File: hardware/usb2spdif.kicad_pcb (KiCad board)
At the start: 2 copper layers, 23 x 20.5 mm, 18 parts, among them J1 USB_C_Receptacle_USB2.0_16P, U1 RP2040, U2 W25Q16JVSS, U3 AP130-33Y, Y1 12MHz

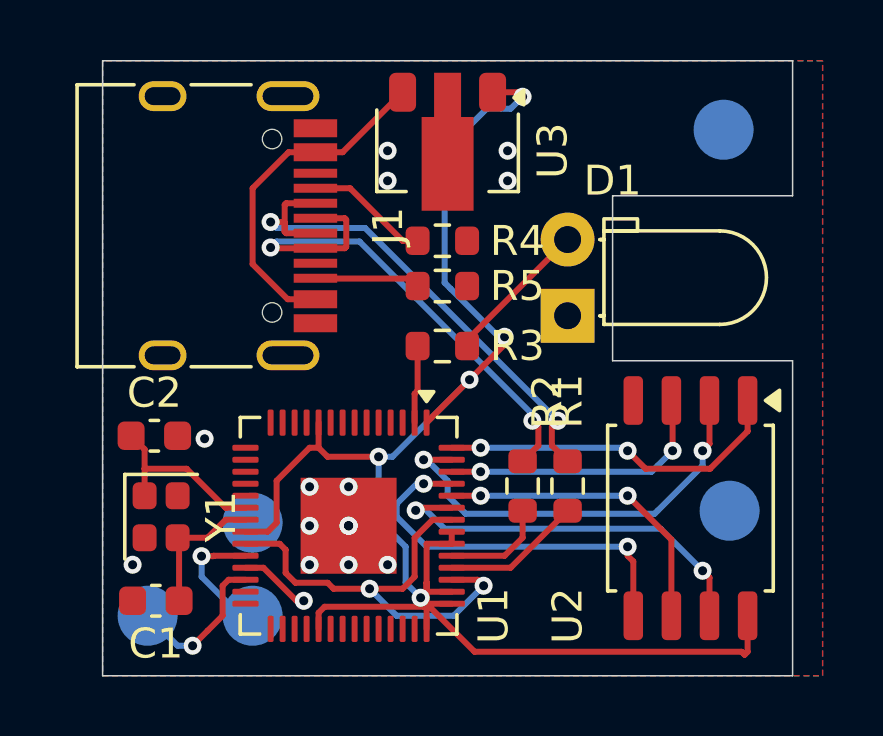
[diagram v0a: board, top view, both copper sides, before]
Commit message: [PCB] minor adjustments
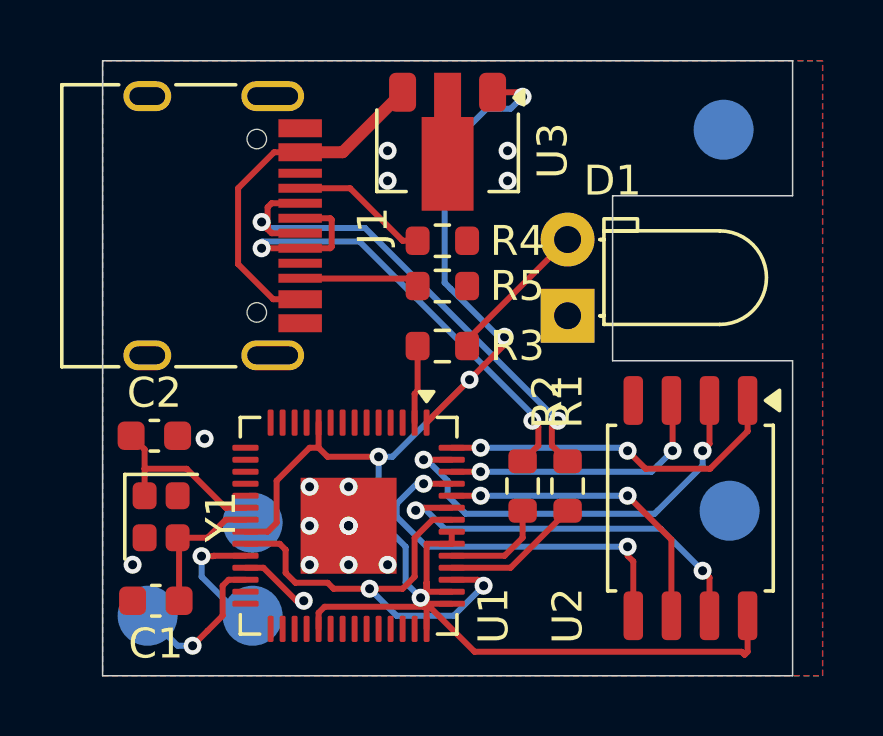
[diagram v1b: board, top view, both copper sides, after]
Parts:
- moved J1 0.51 mm to (23.5, 25.5)
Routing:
- net D-: track 17.7 -> 18.3 mm
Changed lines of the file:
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@@
 	(footprint "Connector_USB:USB_C_Receptacle_HRO_TYPE-C-31-M-12"
 		(layer "F.Cu")
-		(at 24.05 25.5 -90)
+		(at 23.54 25.5 -90)
 		(descr "USB Type-C receptacle for USB 2.0 and PD, http://www.krhro.com/uploads/soft/180320/1-1P320120243.pdf")
 		(tags "usb usb-c 2.0 pd")
@@
 		)
 		(embedded_fonts no)
-		(model "${KICAD9_3DMODEL_DIR}/Connector_USB.3dshapes/USB_C_Receptacle_HRO_TYPE-C-31-M-12.step"
+		(model "${KICAD9_3DMODEL_DIR}/Connector_USB.3dshapes/USB_C_Receptacle_GCT_USB4105-xx-A_16P_TopMnt_Horizontal.step"
 			(offset
 				(xyz 0 0 0)
@@
 			)
 			(rotate
-				(xyz 0 0 0)
+				(xyz -0 -0 -0)
 			)
 		)
@@
 		)
 		(embedded_fonts no)
-		(model "${KICAD9_3DMODEL_DIR}/LED_THT.3dshapes/LED_D3.0mm_Clear.step"
+		(model "${KICAD9_3DMODEL_DIR}/LED_THT.3dshapes/LED_D3.0mm_Horizontal_O1.27mm_Z2.0mm_Clear.step"
 			(offset
-				(xyz 0 1.5 -0.5)
+				(xyz 0 0 -1.5)
 			)
 			(scale
@@
 			)
 			(rotate
-				(xyz -90 -0 -0)
+				(xyz -0 -0 -0)
 			)
 		)
@@
 	)
 	(segment
-		(start 27.069 24.799)
-		(end 27.069 25.701)
+		(start 26.5 25.4355)
+		(end 26.5 25.6155)
 		(width 0.2)
 		(layer "F.Cu")
@@
 	)
 	(segment
-		(start 27.069 25.4)
-		(end 27.069 25.701)
+		(start 26.5 25.6155)
+		(end 26.559 25.6745)
 		(width 0.2)
 		(layer "F.Cu")
@@
 	)
 	(segment
-		(start 27.118 24.75)
-		(end 27.069 24.799)
+		(start 26.3 25.375)
+		(end 26.4395 25.375)
 		(width 0.2)
 		(layer "F.Cu")
@@
 	)
 	(segment
-		(start 28.095 24.75)
-		(end 27.118 24.75)
+		(start 27.6115 24.75)
+		(end 26.6345 24.75)
+		(width 0.2)
+		(layer "F.Cu")
+		(net 5)
+	)
+	(segment
+		(start 26.4395 25.375)
+		(end 26.5 25.4355)
 		(width 0.2)
 		(layer "F.Cu")
@@
 	)
 	(segment
-		(start 26.6 25.375)
-		(end 27.044 25.375)
+		(start 26.5855 25.701)
+		(end 26.6345 25.75)
 		(width 0.2)
 		(layer "F.Cu")
@@
 	)
 	(segment
-		(start 27.069 25.701)
-		(end 27.118 25.75)
+		(start 26.6345 24.75)
+		(end 26.5 24.8845)
 		(width 0.2)
 		(layer "F.Cu")
@@
 	)
 	(segment
-		(start 27.044 25.375)
-		(end 27.069 25.4)
-		(width 0.2)
-		(layer "F.Cu")
-		(net 5)
-	)
-	(segment
-		(start 27.118 25.75)
-		(end 28.095 25.75)
+		(start 26.6345 25.75)
+		(end 27.6115 25.75)
 		(width 0.2)
 		(layer "F.Cu")
@@
 	)
 	(segment
+		(start 26.5 24.8845)
+		(end 26.5 25.6155)
+		(width 0.2)
+		(layer "F.Cu")
+		(net 5)
+	)
+	(segment
 		(start 35.975001 32.199999)
 		(end 36.175 32)
@@
 	)
 	(via
-		(at 26.6 25.375)
+		(at 26.3 25.375)
 		(size 0.6)
 		(drill 0.3)
@@
 	)
 	(segment
+		(start 26.3 25.5585)
+		(end 26.3 25.375)
+		(width 0.2)
+		(layer "B.Cu")
+		(net 5)
+	)
+	(segment
+		(start 29.749999 25.574999)
+		(end 26.316499 25.574999)
+		(width 0.2)
+		(layer "B.Cu")
+		(net 5)
+	)
+	(segment
+		(start 26.316499 25.574999)
+		(end 26.3 25.5585)
+		(width 0.2)
+		(layer "B.Cu")
+		(net 5)
+	)
+	(segment
 		(start 36.175 32)
 		(end 29.749999 25.574999)
@@
 	)
 	(segment
-		(start 26.799999 25.574999)
-		(end 26.6 25.375)
+		(start 26.316499 25.574999)
+		(end 26.799999 25.574999)
 		(width 0.2)
 		(layer "B.Cu")
@@
 	)
 	(segment
-		(start 29.749999 25.574999)
-		(end 26.799999 25.574999)
-		(width 0.2)
-		(layer "B.Cu")
-		(net 5)
-	)
-	(segment
-		(start 28.095 23.05)
-		(end 29 23.05)
-		(width 0.2)
-		(layer "F.Cu")
-		(net 6)
-	)
-	(segment
 		(start 29 23.05)
 		(end 31 21.05)
-		(width 0.2)
+		(width 0.4)
 		(layer "F.Cu")
 		(net 6)
 	)
 	(segment
-		(start 26 24.25)
-		(end 27.2 23.05)
+		(start 25.5165 26.78)
+		(end 25.5165 24.25)
 		(width 0.2)
 		(layer "F.Cu")
@@
 	)
 	(segment
-		(start 26 26.78)
-		(end 26 24.25)
+		(start 26.7165 23.05)
+		(end 27.7 23.05)
 		(width 0.2)
 		(layer "F.Cu")
@@
 	)
 	(segment
-		(start 27.2 23.05)
-		(end 28.095 23.05)
+		(start 26.6865 27.95)
+		(end 25.5165 26.78)
 		(width 0.2)
 		(layer "F.Cu")
@@
 	)
 	(segment
-		(start 28.095 27.95)
-		(end 27.17 27.95)
-		(width 0.2)
+		(start 27.7 23.05)
+		(end 29 23.05)
+		(width 0.4)
 		(layer "F.Cu")
 		(net 6)
 	)
 	(segment
-		(start 27.17 27.95)
-		(end 26 26.78)
+		(start 25.5165 24.25)
+		(end 26.7165 23.05)
 		(width 0.2)
 		(layer "F.Cu")
@@
 	)
 	(segment
-		(start 28.105 27.26)
-		(end 28.095 27.25)
+		(start 27.6115 27.95)
+		(end 26.6865 27.95)
+		(width 0.2)
+		(layer "F.Cu")
+		(net 6)
+	)
+	(segment
+		(start 27.6215 27.26)
+		(end 27.6115 27.25)
 		(width 0.2)
 		(layer "F.Cu")
@@
 	)
 	(segment
-		(start 29.121 25.299)
-		(end 29.072 25.25)
+		(start 28.5885 25.25)
+		(end 27.6115 25.25)
 		(width 0.2)
 		(layer "F.Cu")
@@
 	)
 	(segment
-		(start 29.072 26.25)
-		(end 29.121 26.201)
-		(width 0.2)
-		(layer "F.Cu")
-		(net 8)
-	)
-	(segment
-		(start 28.095 26.25)
-		(end 29.072 26.25)
+		(start 26.3 26.25)
+		(end 28.5885 26.25)
 		(width 0.2)
 		(layer "F.Cu")
@@
 	)
 	(segment
-		(start 28.095 26.25)
-		(end 26.625 26.25)
+		(start 28.6375 26.201)
+		(end 28.6375 25.299)
 		(width 0.2)
 		(layer "F.Cu")
@@
 	)
 	(segment
-		(start 29.121 26.201)
-		(end 29.121 25.299)
+		(start 28.5885 26.25)
+		(end 28.6375 26.201)
 		(width 0.2)
 		(layer "F.Cu")
@@
 	)
 	(segment
-		(start 29.072 25.25)
-		(end 28.095 25.25)
+		(start 28.6375 25.299)
+		(end 28.5885 25.25)
 		(width 0.2)
 		(layer "F.Cu")
 		(net 8)
 	)
-	(segment
-		(start 26.625 26.25)
-		(end 26.6 26.225)
-		(width 0.2)
-		(layer "F.Cu")
-		(net 8)
-	)
 	(via
-		(at 26.6 26.225)
+		(at 26.3 26.25)
 		(size 0.6)
 		(drill 0.3)
@@
 	)
 	(segment
-		(start 35.325 31.786397)
-		(end 29.563604 26.025001)
+		(start 26.3 26.25)
+		(end 26.3 26.0415)
 		(width 0.2)
 		(layer "B.Cu")
@@
 	)
 	(segment
-		(start 35.325 32)
+		(start 29.563604 26.025001)
 		(end 35.325 31.786397)
 		(width 0.2)
@@
 	)
 	(segment
-		(start 29.563604 26.025001)
-		(end 26.799999 26.025001)
+		(start 26.3 26.0415)
+		(end 26.316499 26.025001)
 		(width 0.2)
 		(layer "B.Cu")
@@
 	)
 	(segment
-		(start 26.799999 26.025001)
-		(end 26.6 26.225)
+		(start 26.316499 26.025001)
+		(end 29.563604 26.025001)
+		(width 0.2)
+		(layer "B.Cu")
+		(net 8)
+	)
+	(segment
+		(start 35.325 31.786397)
+		(end 35.325 32)
 		(width 0.2)
 		(layer "B.Cu")
@@
 	(segment
 		(start 29.25 24.25)
-		(end 28.095 24.25)
-		(width 0.2)
-		(layer "F.Cu")
+		(end 27.6115 24.25)
+		(width 0.2)
+		(layer "F.Cu")
